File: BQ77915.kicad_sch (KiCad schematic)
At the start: 1 part, among them U1 BQ7791500PWR

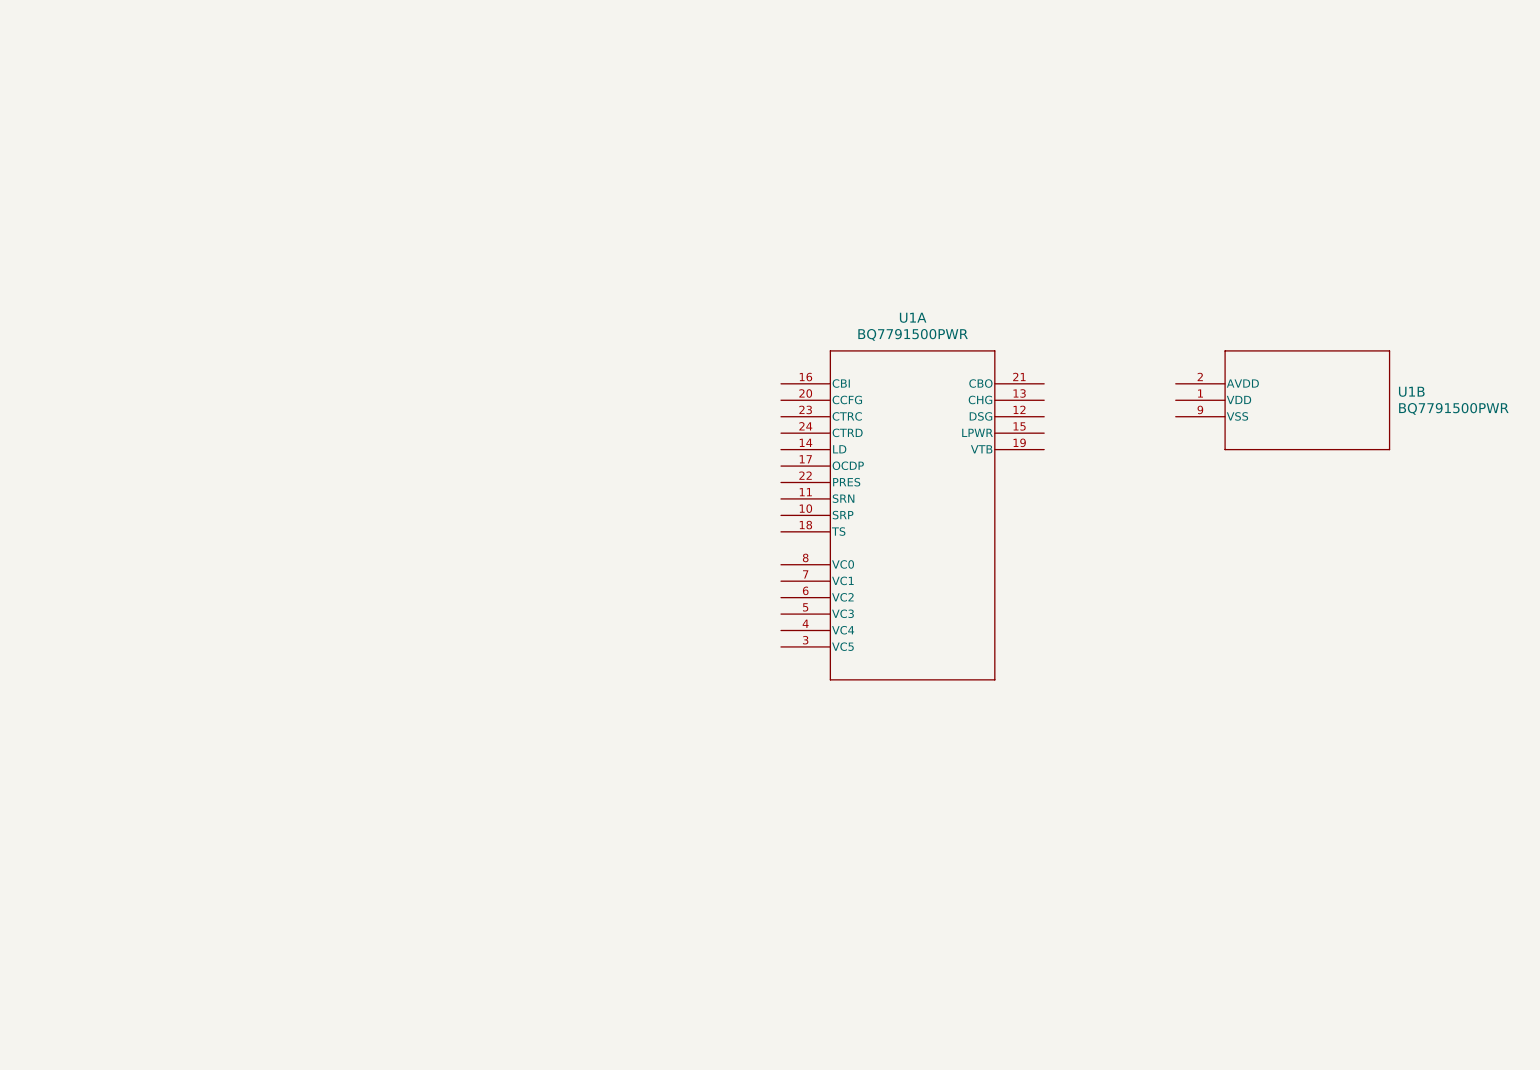
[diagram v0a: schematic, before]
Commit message: added SA balancer design (WiP)
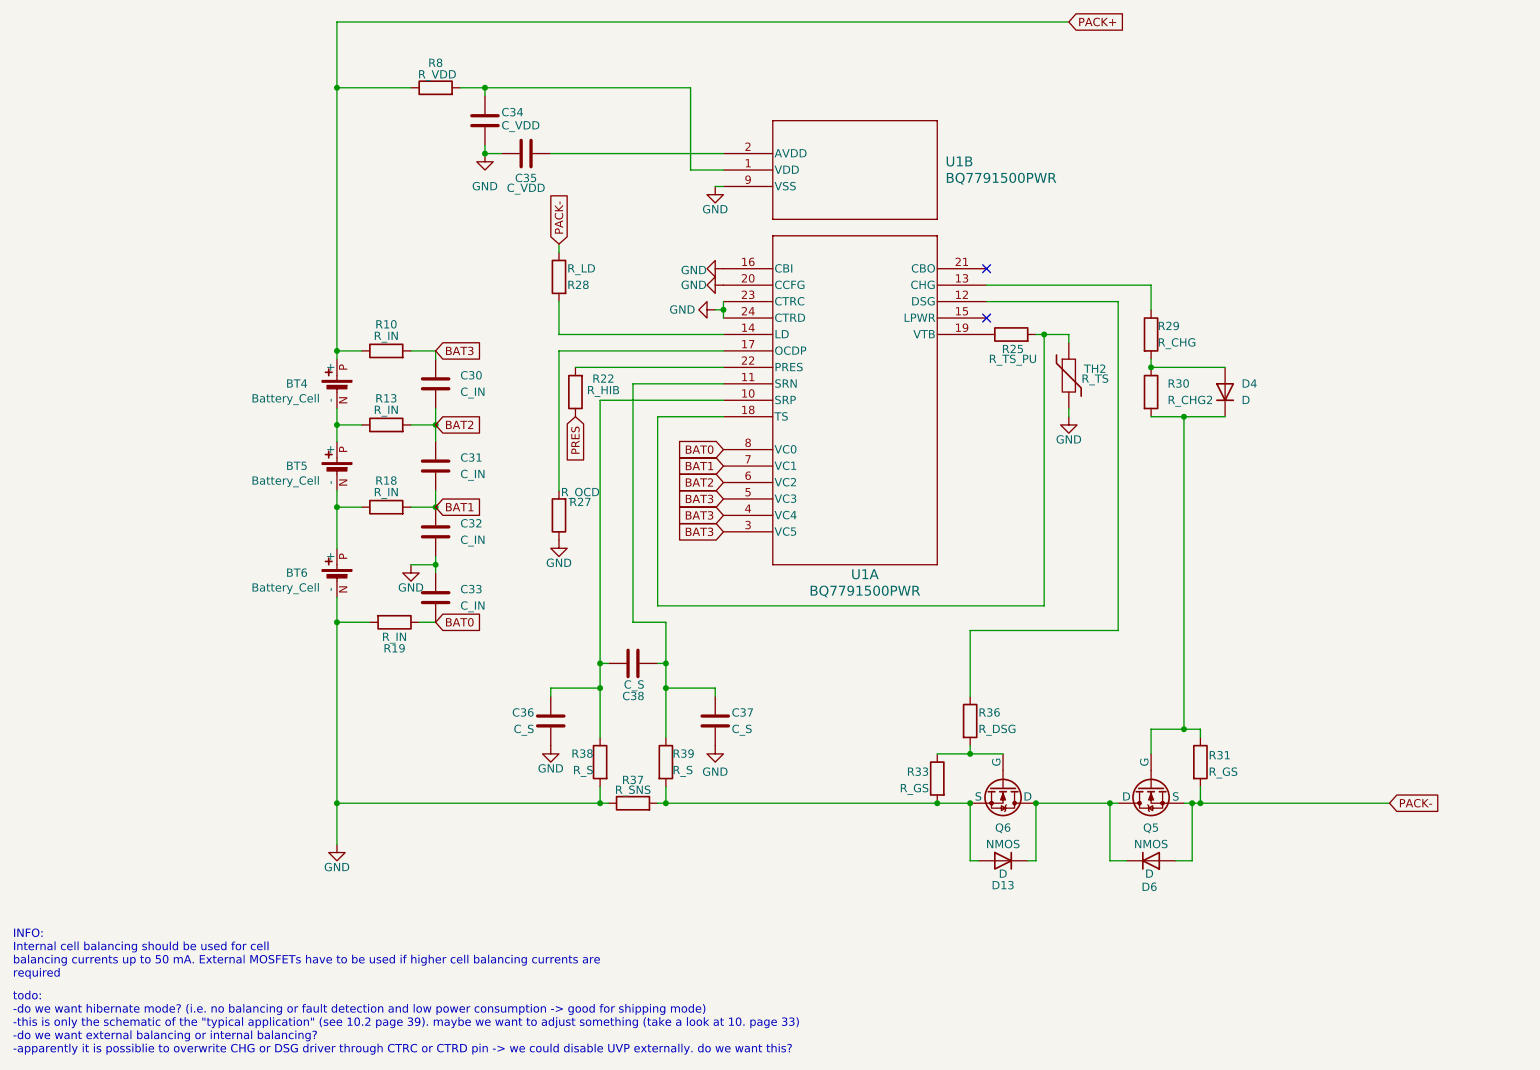
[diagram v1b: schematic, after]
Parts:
- added BT4, BT5, BT6: Battery_Cell, Inductor Wuerth:BAT_1043, symbol Device:Battery_Cell
- added C30, C31, C32, C33: C_IN, symbol Device:C
- added C34, C35: C_VDD, symbol Device:C
- added C36, C37, C38: C_S, symbol Device:C
- added D13, D4, D6: D, symbol Device:D
- added Q5, Q6: NMOS, symbol Simulation_SPICE:NMOS
- added R10, R13, R18, R19: R_IN, symbol Device:R
- added R22: R_HIB, symbol Device:R
- added R25: R_TS_PU, symbol Device:R
- added R27: R_OCD, symbol Device:R
- added R28: R_LD, symbol Device:R
- added R29: R_CHG, symbol Device:R
- added R30: R_CHG2, symbol Device:R
- added R31, R33: R_GS, symbol Device:R
- added R36: R_DSG, symbol Device:R
- added R37: R_SNS, symbol Device:R
- added R38, R39: R_S, symbol Device:R
- added R8: R_VDD, symbol Device:R
- added TH2: R_TS, symbol Device:Thermistor
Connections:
- net at U1.1 (VDD): now also C34.1, R8.2
- net at U1.2 (AVDD): now also C35.1
- net GND: now reaches U1.9 (VSS)
- net GND: now also U1.16 (CBI), U1.20 (CCFG), U1.23 (CTRC), U1.24 (CTRD), BT6.N (-), C32.2, C33.1, C34.2, C35.2, C36.2, C37.2, R19.2, R27.1, R37.1, R38.2, TH2.2
- net at U1.10 (SRP): now also C36.1, C38.1, R38.1
- net at U1.11 (SRN): now also C37.1, C38.2, R39.1
- net at U1.12 (DSG): now also R36.1
- net at U1.13 (CHG): now also R29.1
- net at U1.14 (LD): now also R28.2
- net at U1.17 (OCDP): now also R27.2
- net at U1.18 (TS): now also R25.2, TH2.1
- net at U1.19 (VTB): now also R25.1
- net at U1.22 (PRES): now also R22.2
- net BAT3: now reaches U1.3 (VC5)
- net BAT3: now also U1.4 (VC4), U1.5 (VC3), C30.1, R10.2
- net BAT2: now reaches U1.6 (VC2)
- net BAT2: now also C30.2, C31.1, R13.2
- net BAT1: now reaches U1.7 (VC1)
- net BAT1: now also C31.2, C32.1, R18.2
- net BAT0: now reaches U1.8 (VC0)
- net BAT0: now also C33.2, R19.1
- new net: D4.1 (K), Q5.2 (G), R30.2, R31.1
- new net: D4.2 (A), R29.2, R30.1
- new net: Q6.2 (G), R33.1, R36.2
- new net: D13.1 (K), D6.1 (K), Q5.1 (D), Q6.1 (D)
- new net: D13.2 (A), Q6.3 (S), R33.2, R37.2, R39.2
- new net: BT5.N (-), BT6.P (+), R18.1
- new net: BT4.N (-), BT5.P (+), R13.1
- new net PACK+: BT4.P (+), R10.1, R8.1
- new net PACK-: D6.2 (A), Q5.3 (S), R28.1, R31.2
- new net PRES: R22.1
- no-connect marks 0 -> 2
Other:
- note added: "INFO: Internal cell balancing should be used for cell balancing currents up to 50 mA. External MOSFETs have to be used if higher cell balancing currents are required"
- note added: "todo: -do we want hibernate mode? (i.e. no balancing or fault detection and low power consumption -> good for shipping mode) -this is only the schematic of the "typical application" (see 10.2 page 39). maybe we want to adjust something (take a look at 10. page 33) -do we want external balancing or internal balancing? -apparently it is possiblie to overwrite CHG or DSG driver through CTRC or CTRD 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"
- moved on the sheet: U1A, U1B
